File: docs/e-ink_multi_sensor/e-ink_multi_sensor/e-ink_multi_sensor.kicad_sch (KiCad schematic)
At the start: 5 parts, among them J1 HC-SR501, J2 SCD41, J3 BME280, U1 ESP32-S3-DevKitC

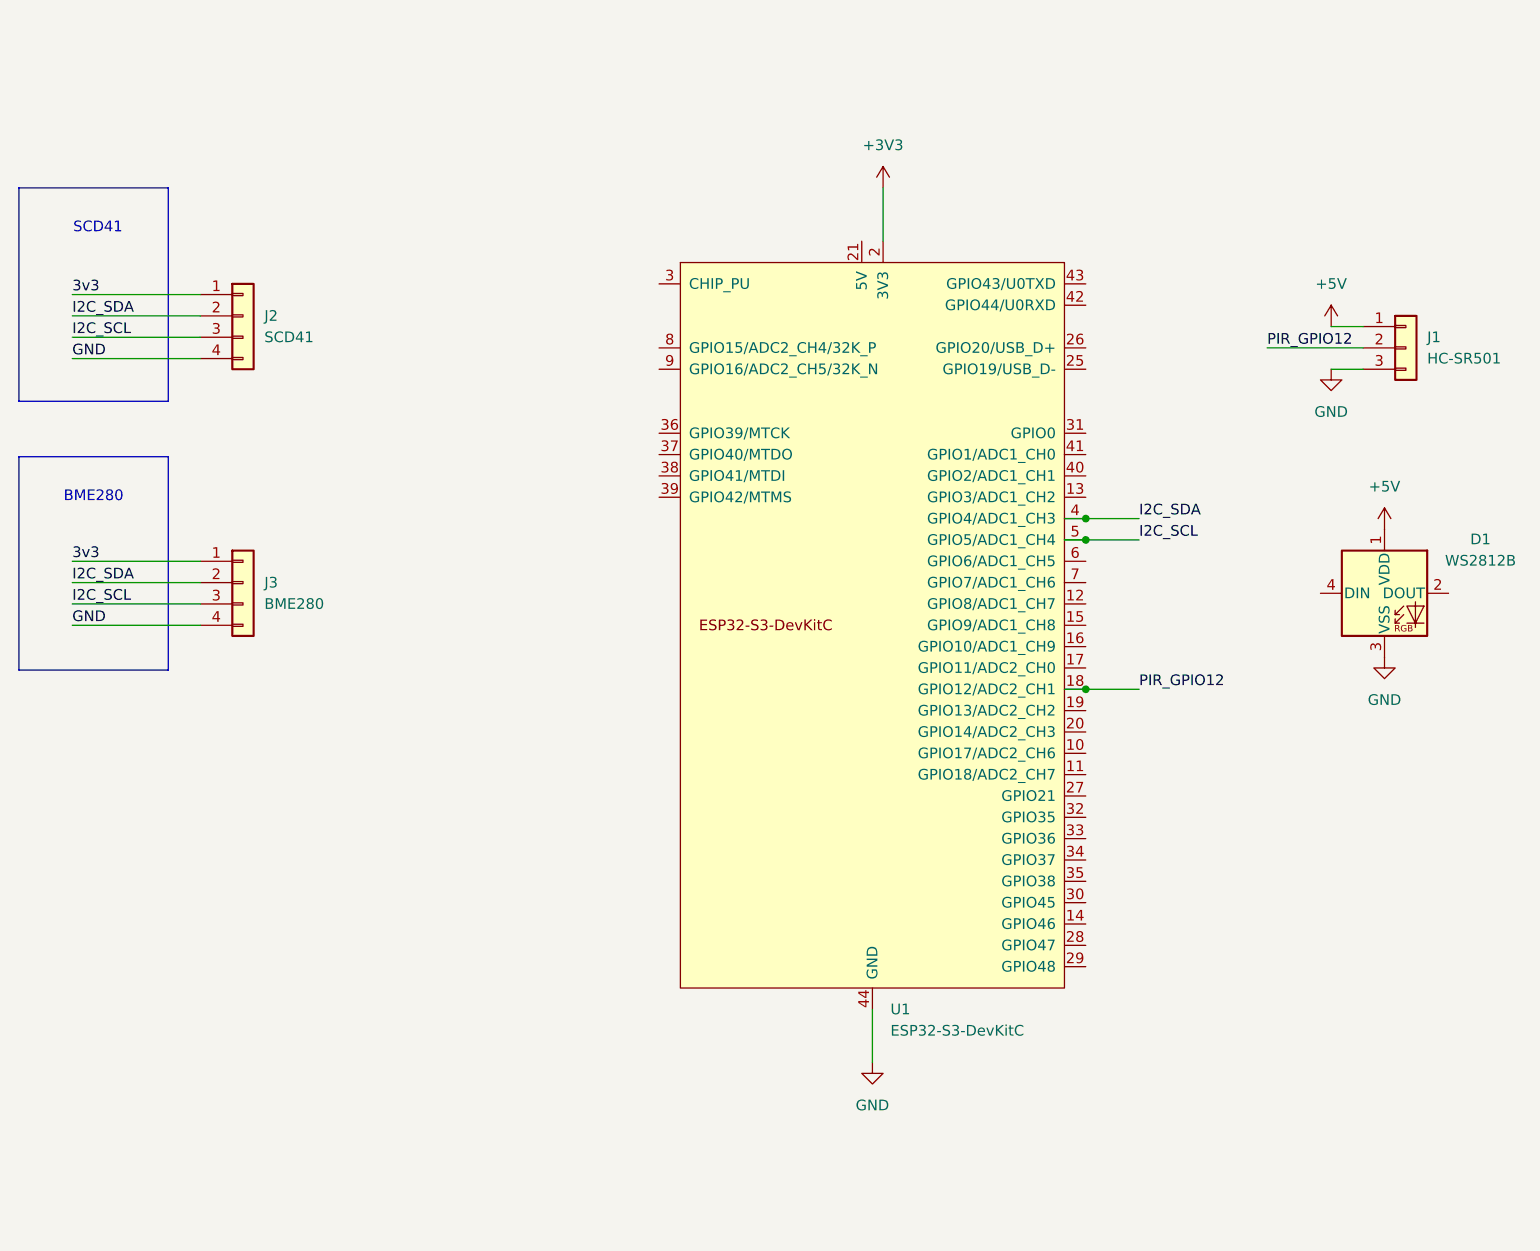
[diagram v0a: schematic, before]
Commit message: schematic
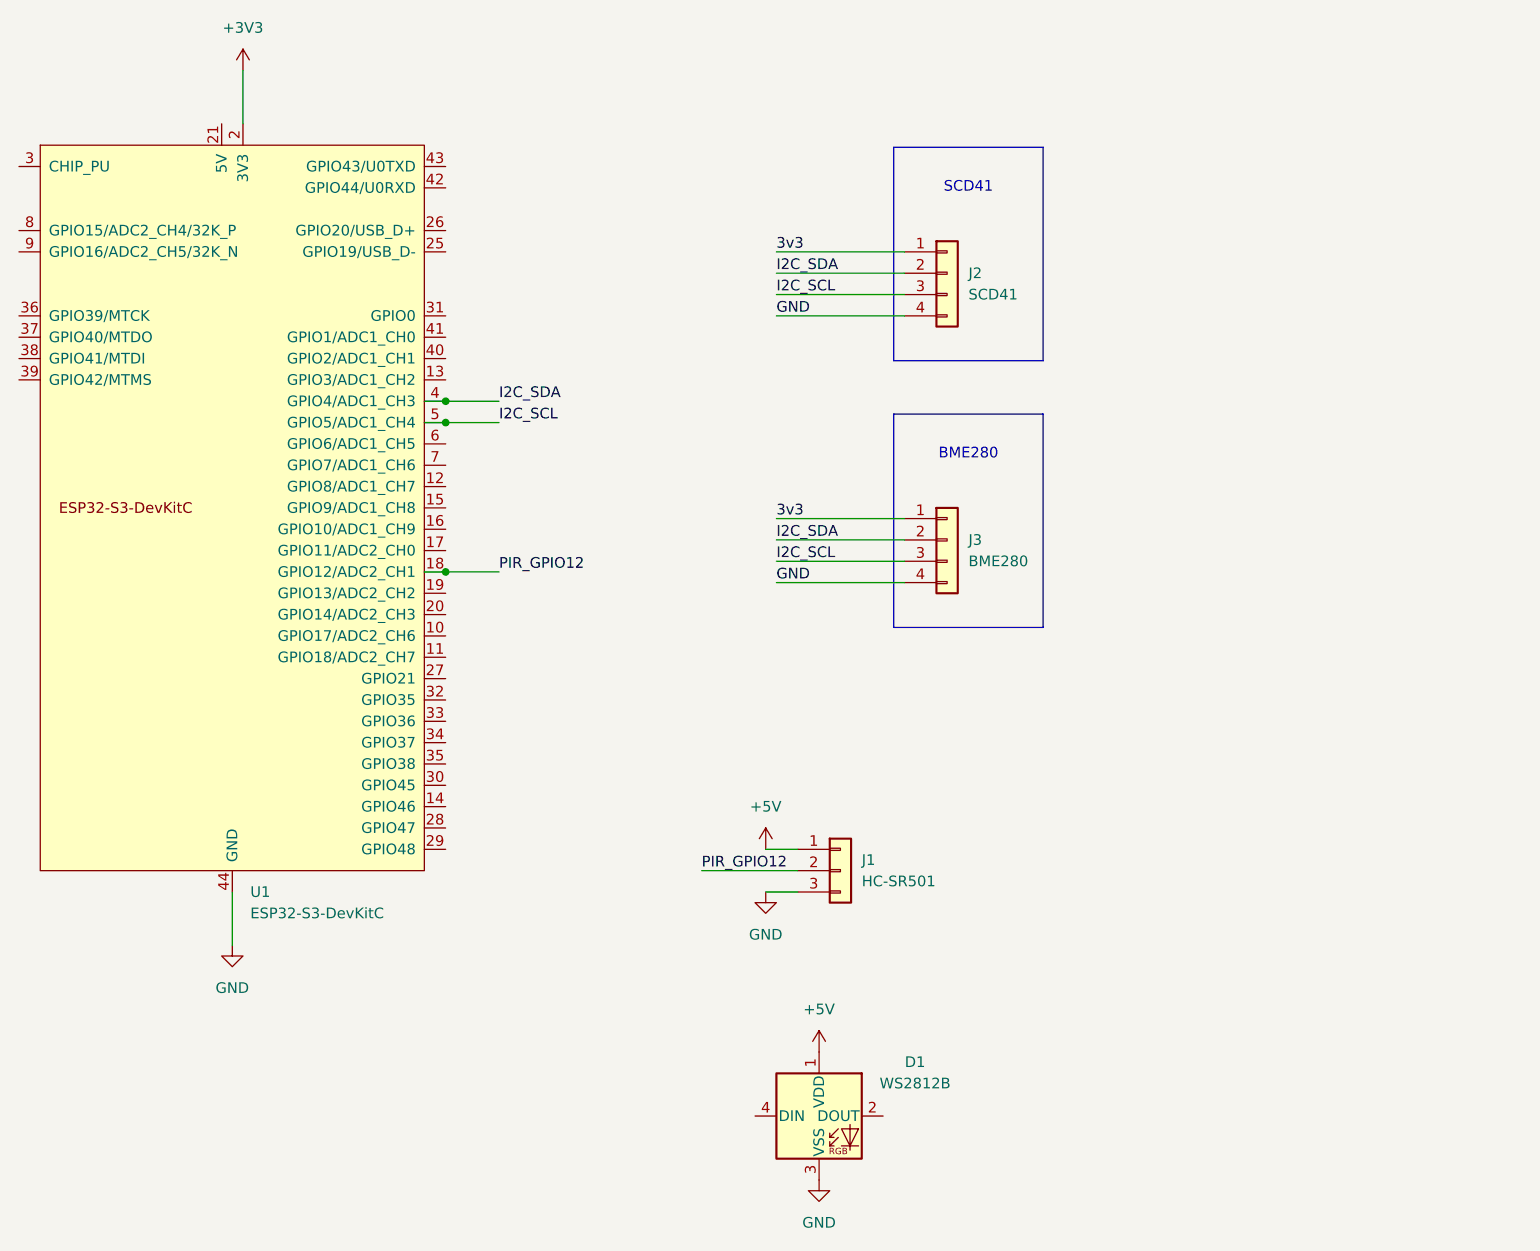
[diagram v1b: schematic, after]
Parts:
- J1: footprint Sensor:Sensirion_SCD4x-1EP_10.1x10.1mm_P1.25mm_EP4.8x4.8mm -> Connector_JST:JST_EH_B3B-EH-A_1x03_P2.50mm_Vertical
- J2, J3: footprint PCM_Espressif:ESP32-S3-DevKitC -> Connector:NS-Tech_Grove_1x04_P2mm_Vertical
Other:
- title: (none) -> Multi-sensor ESP32 board with e-ink display
- moved on the sheet: D1, J1, J2, J3, U1
